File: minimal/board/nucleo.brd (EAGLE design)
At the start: 22.9 x 38.1 mm, 9 parts

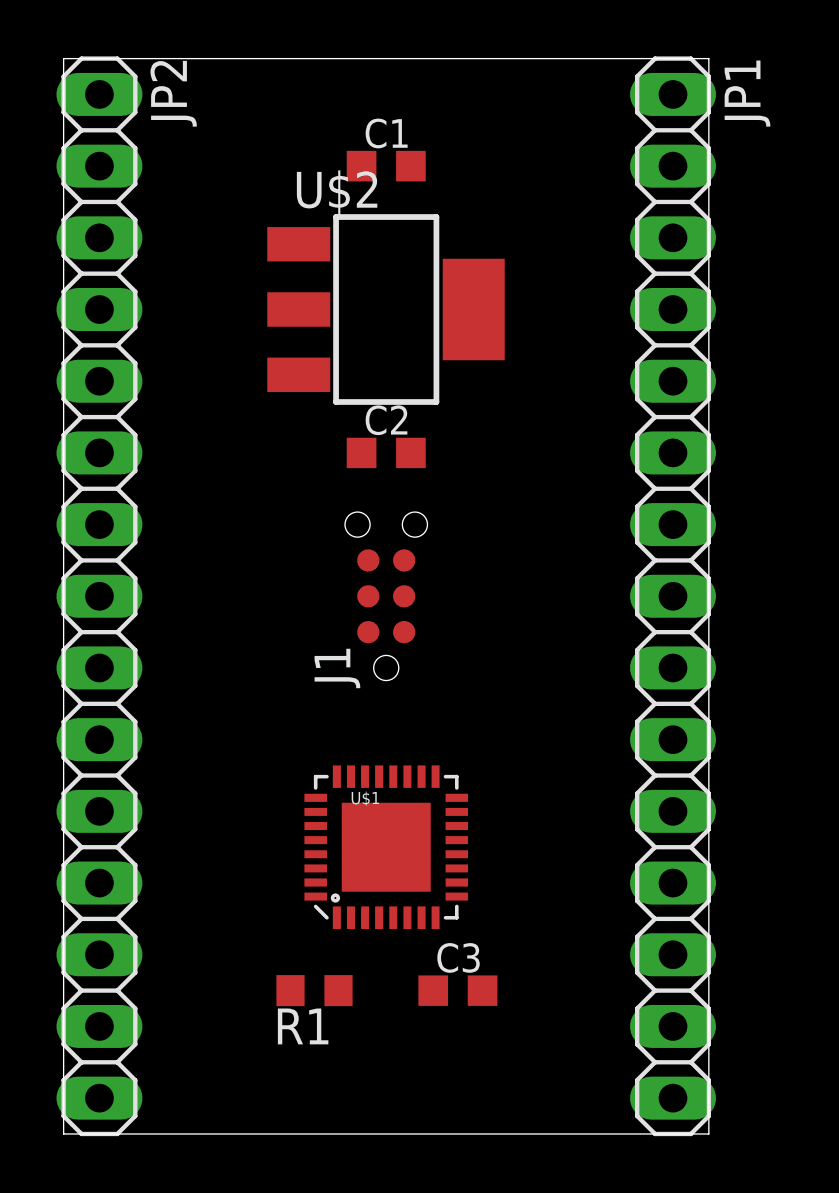
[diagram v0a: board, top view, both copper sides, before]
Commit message: updates from Austin through Aug 2017
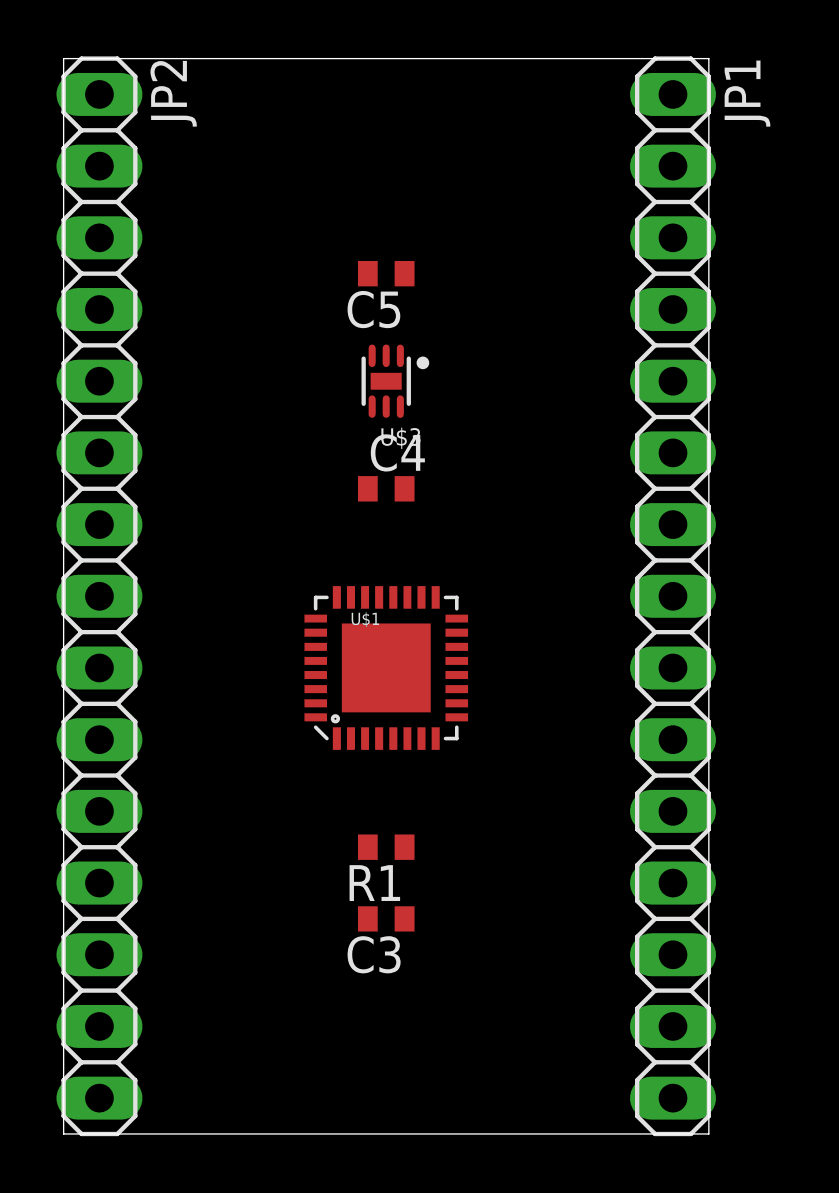
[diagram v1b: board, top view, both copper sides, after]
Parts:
- removed C1: 0.1uF, rcl:C0603K
- removed C2: 1uF, rcl:C0603K
- removed J1: (no value), modular_robotics:TAG-CONNECT_TC2030-MCP-NL
- removed U$2: TC1262, modular_robotics:SOT223
- added C4, C5: 2.2uF, rcl:C0402
- added U$3: MIC5305-MLF, modular_robotics:MLF-6
- C3: device rcl:C0603K -> rcl:C0402
- R1: device rcl:R0603 -> rcl:R0402
- moved U$1 6.35 mm to (11.4, 16.5)
- moved R1 5.68 mm to (11.4, 10.2)
- moved C3 3.59 mm to (11.4, 7.62), turned to 180 degrees
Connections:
- net +3V3: now also C4.1, U$3.4; no longer C2.1, J1.1, U$2.3
- net GND: now also C4.2, C5.2, U$3.2; no longer C1.2, C2.2, J1.5, U$2.2
- net NRST: no longer J1.3
- net PA13: no longer J1.2
- net PA14: no longer J1.4
- net VCC: now also C5.1, U$3.1, U$3.3; no longer C1.1, U$2.1
